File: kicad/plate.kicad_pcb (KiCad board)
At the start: 2 copper layers, 123.5 x 85.3 mm, 22 parts, among them J1 TRRS, SW10 SW_PUSH, SW11 SW_PUSH, SW12 SW_PUSH, SW14 SW_PUSH, SW15 SW_PUSH, SW16 SW_PUSH, SW17 SW_PUSH, SW18 SW_PUSH, SW2 SW_PUSH, SW20 SW_PUSH, SW21 SW_PUSH, SW3 SW_PUSH, SW4 SW_PUSH, SW5 SW_PUSH, SW6 SW_PUSH, SW8 SW_PUSH, SW9 SW_PUSH, U1 ProMicro

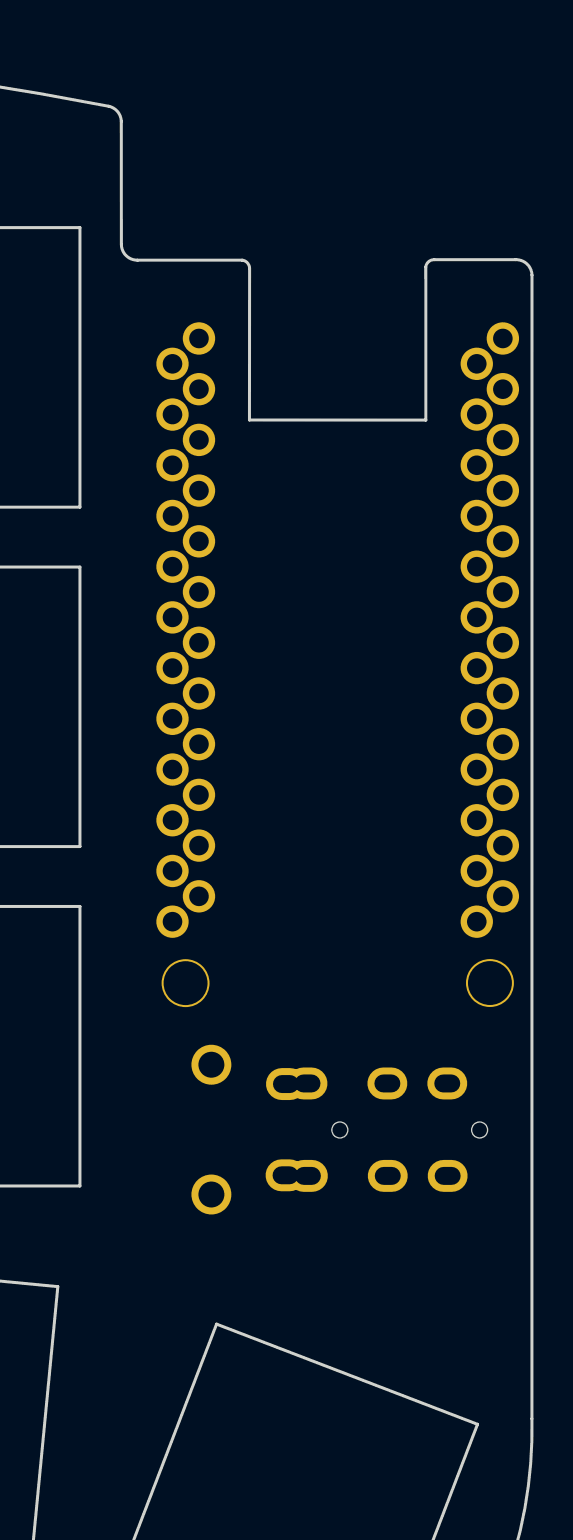
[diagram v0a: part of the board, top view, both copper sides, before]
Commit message: Plate ready
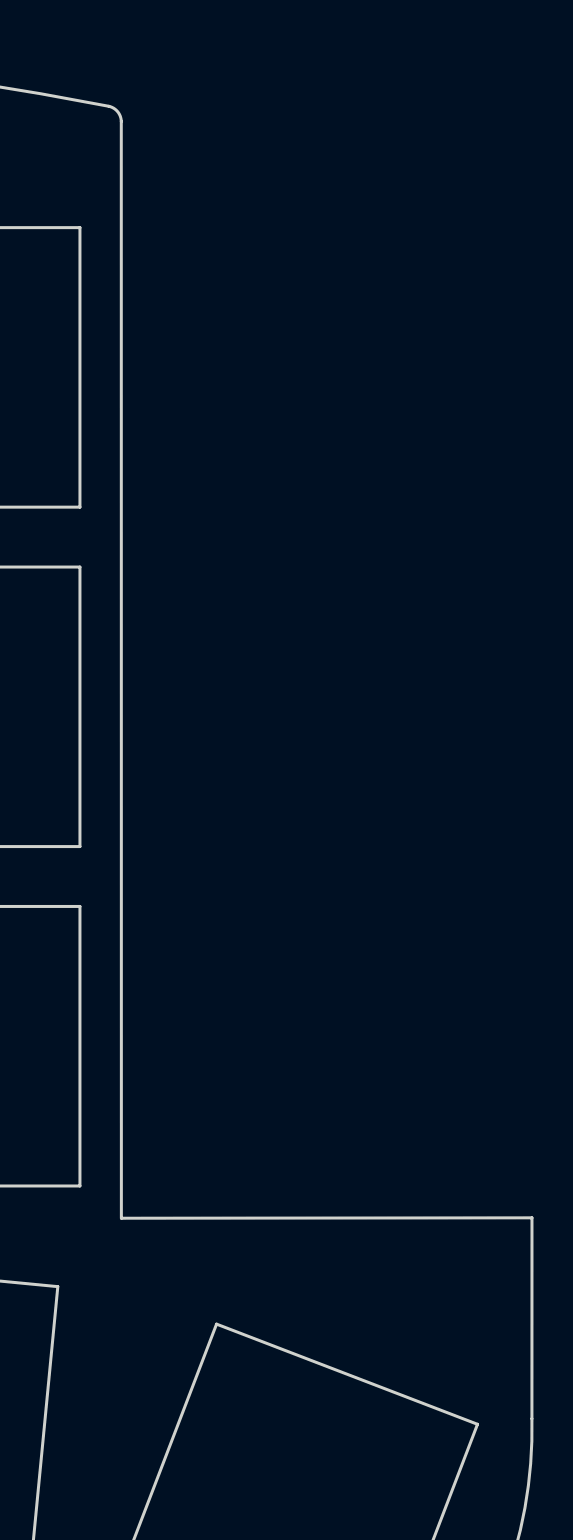
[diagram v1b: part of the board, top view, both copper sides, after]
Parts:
- removed J1: TRRS, broom:TRRS-PJ-DPB2
- removed RSW1: Val**, foostan:ResetSW
- removed U1: ProMicro, broom:ProMicro_v2
- removed h2 (x2): h2, chocorne:LEGO_HOLE
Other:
- outline, holes or cut-outs redrawn
